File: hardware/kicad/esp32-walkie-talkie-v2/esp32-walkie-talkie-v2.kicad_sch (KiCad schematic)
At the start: 21 parts, among them J1 inmp441 left, J2 inmp441 right, J3 ST7789, J4 extend, J5 POWER_IN_5V, J6 MAX98357, J7 Transimit switch, P1 Power, P2 Analog, P3 Digital, P4 Digital, P5 CONN_01X01, P6 CONN_01X01, P7 CONN_01X01, P8 CONN_01X01

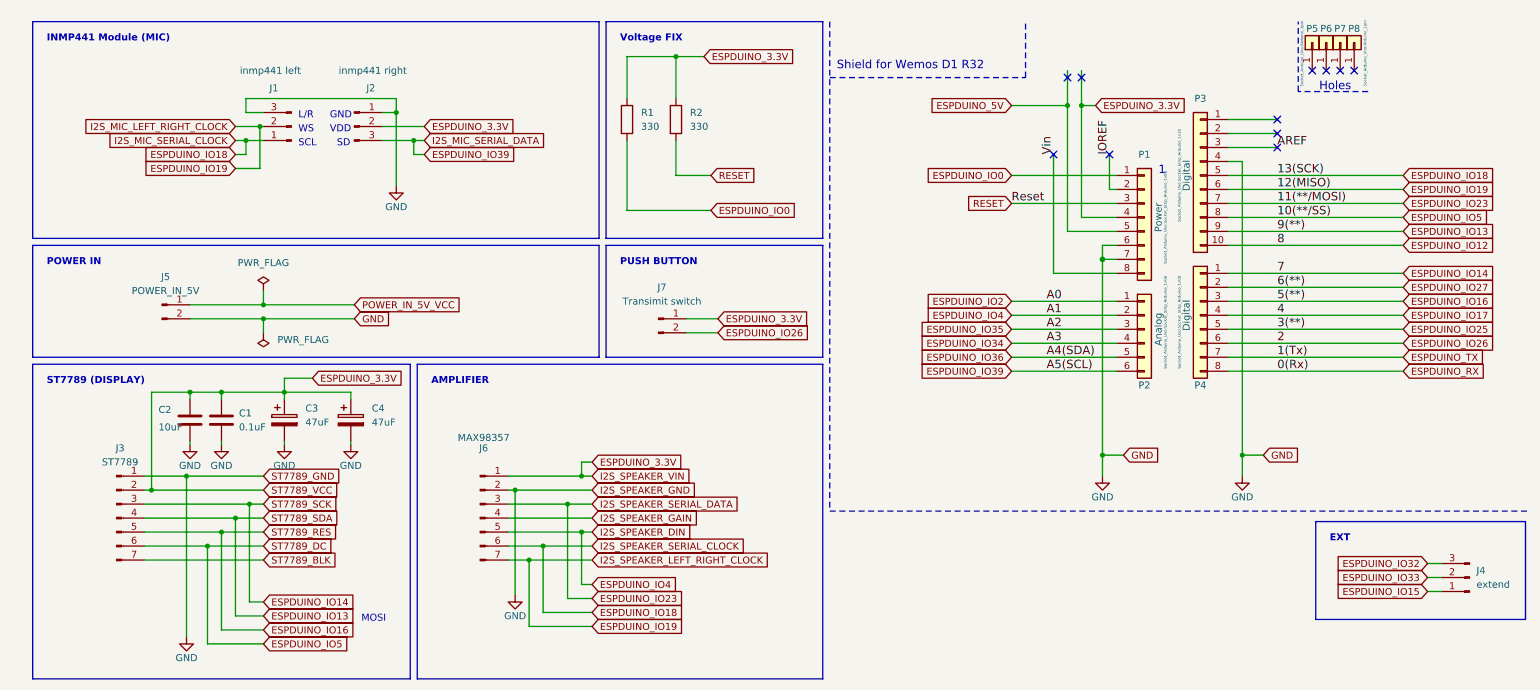
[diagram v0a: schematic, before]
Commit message: add text, new copper fill
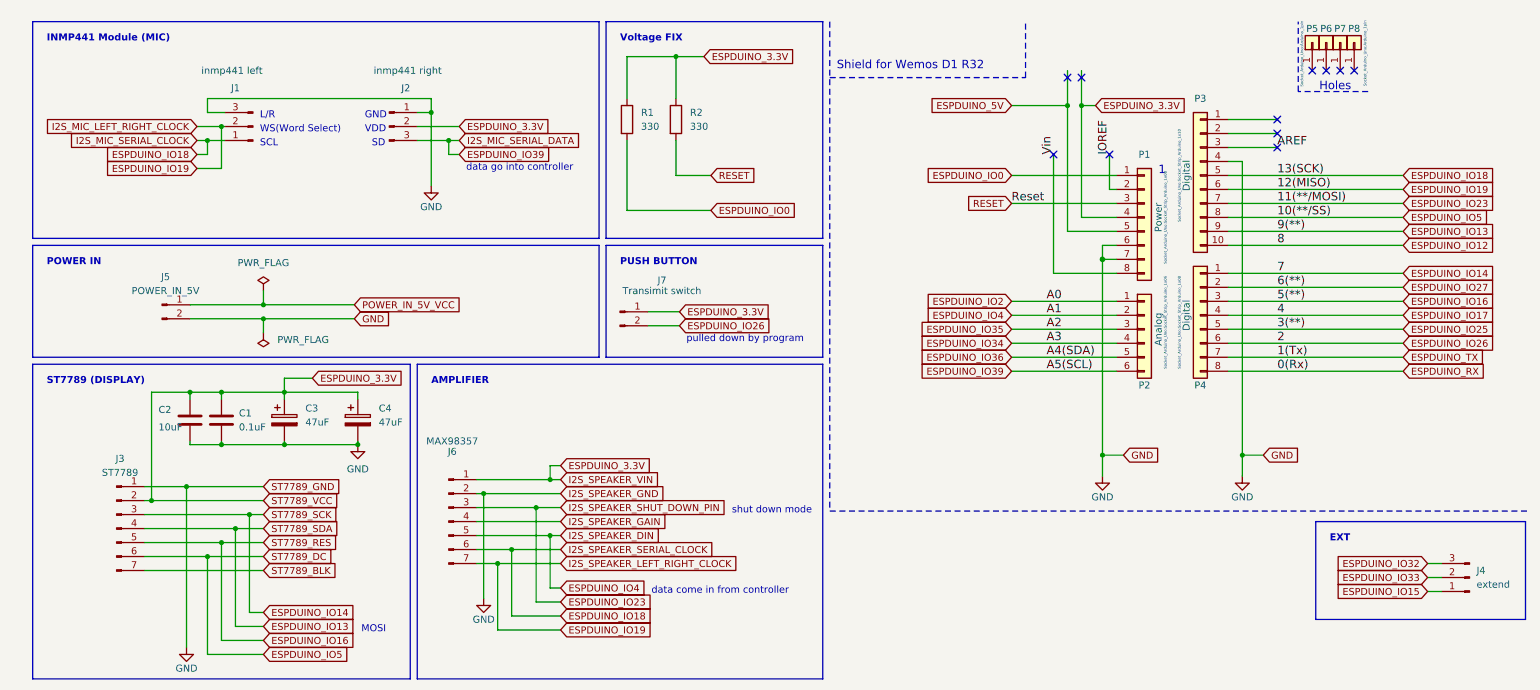
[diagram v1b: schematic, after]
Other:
- note added: "WS(Word Select)"
- note added: "data come in from controller"
- note added: "data go into controller"
- note added: "pulled down by program"
- note added: "shut down mode"
- note removed: "WS"
- moved on the sheet: C4, J1, J2, J3, J6, J7

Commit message: update
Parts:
- R1, R2: footprint Resistor_SMD:R_0603_1608Metric -> Resistor_SMD:R_1206_3216Metric
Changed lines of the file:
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@@
       (effects (font (size 1.27 1.27)) (justify left))
     )
-    (property "Footprint" "Resistor_SMD:R_0603_1608Metric" (id 2) (at 127.762 30.48 90)
+    (property "Footprint" "Resistor_SMD:R_1206_3216Metric" (id 2) (at 127.762 30.48 90)
       (effects (font (size 1.27 1.27)) hide)
     )
@@
       (effects (font (size 1.27 1.27)) (justify left))
     )
-    (property "Footprint" "Resistor_SMD:R_0603_1608Metric" (id 2) (at 118.872 30.48 90)
+    (property "Footprint" "Resistor_SMD:R_1206_3216Metric" (id 2) (at 118.872 30.48 90)
       (effects (font (size 1.27 1.27)) hide)
     )
@@
     )
     (path "/f67dee4a-805c-4563-ba28-5a6bba1ad765"
-      (reference "R1") (unit 1) (value "330") (footprint "Resistor_SMD:R_0603_1608Metric")
+      (reference "R1") (unit 1) (value "330") (footprint "Resistor_SMD:R_1206_3216Metric")
     )
     (path "/5d57424f-adb7-4874-b837-6a4aae2030e9"
-      (reference "R2") (unit 1) (value "330") (footprint "Resistor_SMD:R_0603_1608Metric")
-    )
-  )
+      (reference "R2") (unit 1) (value "330") (footprint "Resistor_SMD:R_1206_3216Metric")
+    )
+  )
